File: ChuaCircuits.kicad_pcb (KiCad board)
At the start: 2 copper layers, 23 parts, among them J1 BanaJack 9V, J2 BanaJack GND, J3 BanaJack -9V, U1 TL082, U2 TL082

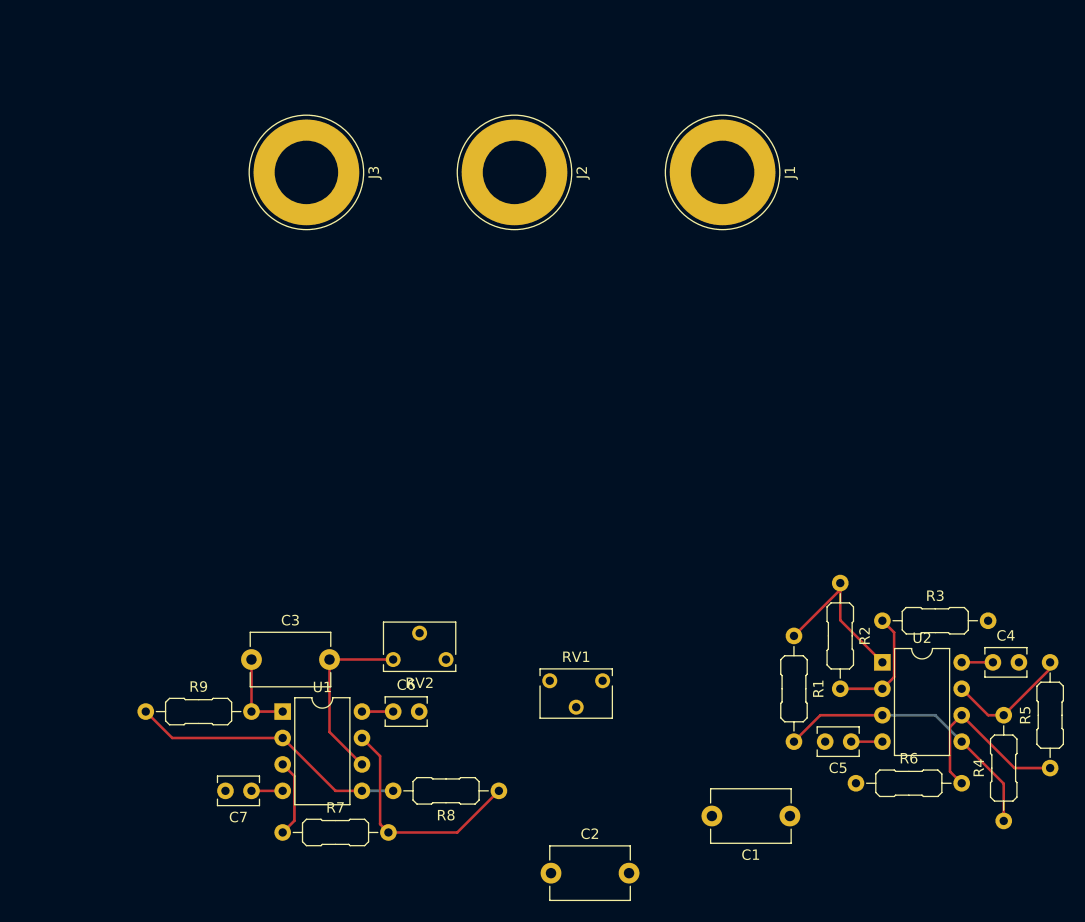
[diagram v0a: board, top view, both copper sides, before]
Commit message: finished board v1
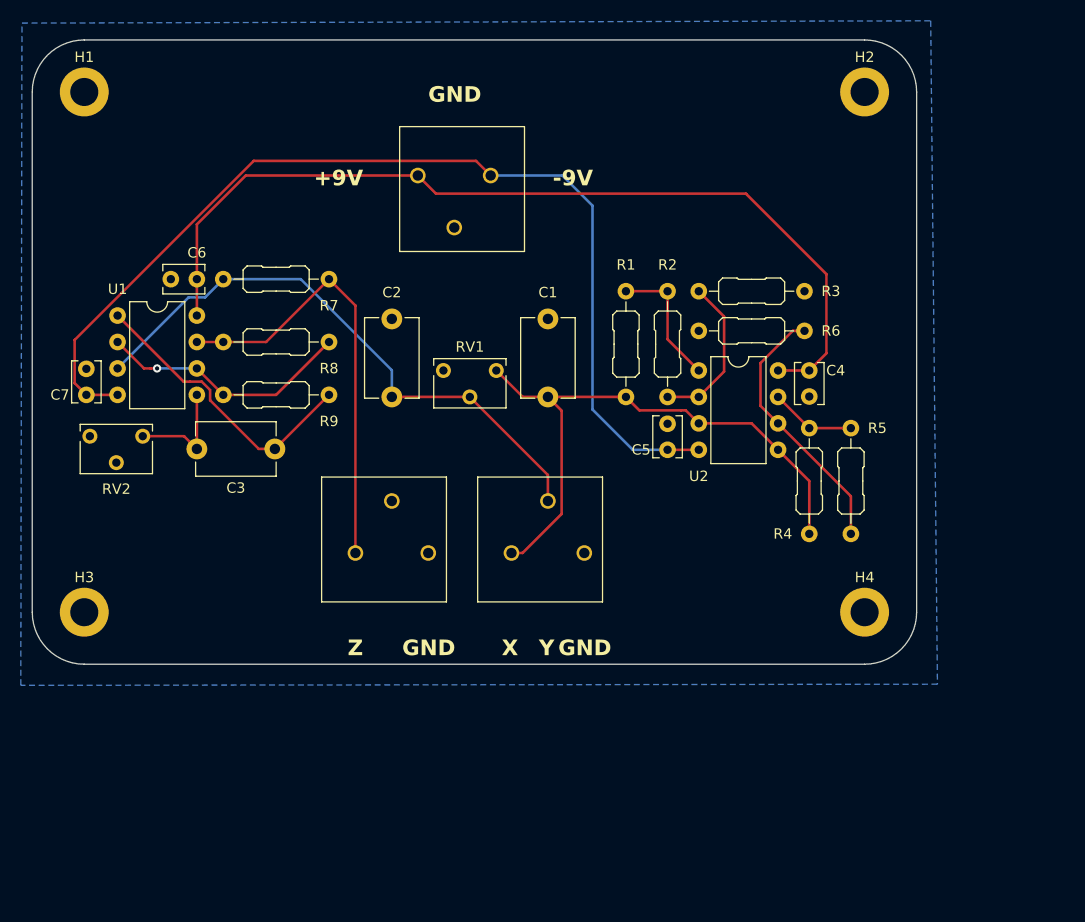
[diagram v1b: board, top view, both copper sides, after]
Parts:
- added H1: MountingHole_Pad, MountingHole:MountingHole_2.7mm_M2.5_DIN965_Pad, F.Cu at (73.6, 66.5)
- added H2: MountingHole_Pad, MountingHole:MountingHole_2.7mm_M2.5_DIN965_Pad, F.Cu at (148.6, 66.5)
- added H3: MountingHole_Pad, MountingHole:MountingHole_2.7mm_M2.5_DIN965_Pad, F.Cu at (73.6, 116.5)
- added H4: MountingHole_Pad, MountingHole:MountingHole_2.7mm_M2.5_DIN965_Pad, F.Cu at (148.6, 116.5)
- J1: value BanaJack 9V -> PWR_Input; footprint Connector:Banana_Jack_1Pin -> addons:1985205
- J2: value BanaJack GND -> Output_1; footprint Connector:Banana_Jack_1Pin -> addons:1985205
- J3: value BanaJack -9V -> Output_1; footprint Connector:Banana_Jack_1Pin -> addons:1985205
- moved R7 53.5 mm to (86.9, 84.5)
- moved R8 50.6 mm to (86.9, 90.6), turned to 0 degrees
- moved C2 48.3 mm to (103.1, 95.8), turned to 90 degrees
- moved C1 46.5 mm to (118.1, 95.8), turned to 90 degrees
- moved R6 46.0 mm to (132.6, 89.5)
- moved C6 45.6 mm to (84.4, 84.5), turned to 180 degrees
- moved U1 41.2 mm to (76.8, 88.0)
- moved C7 41.2 mm to (73.8, 95.6), turned to 90 degrees
- moved R1 36.9 mm to (125.6, 85.7)
- moved R3 36.3 mm to (132.6, 85.7)
- moved J3 36.1 mm to (102.4, 109.5), turned to 0 degrees
- moved J2 35.4 mm to (117.4, 109.5), turned to 0 degrees
- moved R4 33.3 mm to (143.2, 109.0)
- moved C5 33.1 mm to (129.6, 100.9), turned to 90 degrees
- moved U2 33.1 mm to (132.6, 93.3)
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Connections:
- C1 pad 1: Net-(U2A-+) -> /X-Value
- C2 pad 1: Net-(U1A-+) -> /Y-Value
- C3 pad 2: Net-(U1B--) -> Net-(U1B-+)
- J1 pad 1: +9V -> -9V
- J2 pad 1: GND -> /X-Value
- J3 pad 1: -9V -> /Z-Value
- R1 pad 2: Net-(U2A-+) -> /X-Value
- R4 pad 1: Net-(U2A-+) -> /X-Value
- R7 pad 1: Net-(U1A-+) -> /Y-Value
- R7 pad 2: Net-(R7-Pad2) -> /Z-Value
- R8 pad 1: Net-(R7-Pad2) -> /Z-Value
- RV1 pad 1: Net-(U2A-+) -> /X-Value
- RV1 pad 2: Net-(U1A-+) -> /Y-Value
- RV2 pad 1: Net-(U1B--) -> Net-(U1B-+)
- U1 pad 3: Net-(U1A-+) -> /Y-Value
- U1 pad 5: Net-(U1A--) -> Net-(U1B-+)
- U1 pad 6: Net-(U1B--) -> Net-(U1A--)
- U1 pad 7: Net-(R7-Pad2) -> /Z-Value
- U2 pad 3: Net-(U2A-+) -> /X-Value
- U2 pad 5: Net-(U2A-+) -> /X-Value
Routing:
- net -9V: track 6.00 -> 98.8 mm
- net +9V: track 6.00 -> 88.1 mm
- net /X-Value: track 0.00 -> 57.7 mm
- net /Y-Value: track 0.00 -> 56.7 mm
- net /Z-Value: track 0.00 -> 42.6 mm
- net Net-(U2A-+): track 27.5 -> 0.00 mm
- net Net-(R7-Pad2): track 22.4 -> 0.00 mm
- net Net-(C3-Pad1): track 8.00 -> 28.4 mm
- net Net-(U1B--): track 17.5 -> 0.00 mm
- net Net-(U1B-+): track 0.00 -> 10.9 mm
- net Net-(U1A-+): track 7.47 -> 0.00 mm
- net Net-(U2B--): track 18.1 -> 25.5 mm
- net Net-(R4-Pad2): track 12.0 -> 8.24 mm
- net Net-(U2A--): track 11.5 -> 15.2 mm
- net Net-(R1-Pad1): track 16.2 -> 12.9 mm
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- added copper zone on B.Cu, net GND
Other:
- board outline added: 85 x 60 mm
- board text added: "+9V"
- board text added: "-9V"
- board text added: "GND"
- board text added: "X"
- board text added: "Y"
- board text added: "Z"
